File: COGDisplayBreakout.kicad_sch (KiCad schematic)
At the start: 12 parts, among them J2 SPI_Header

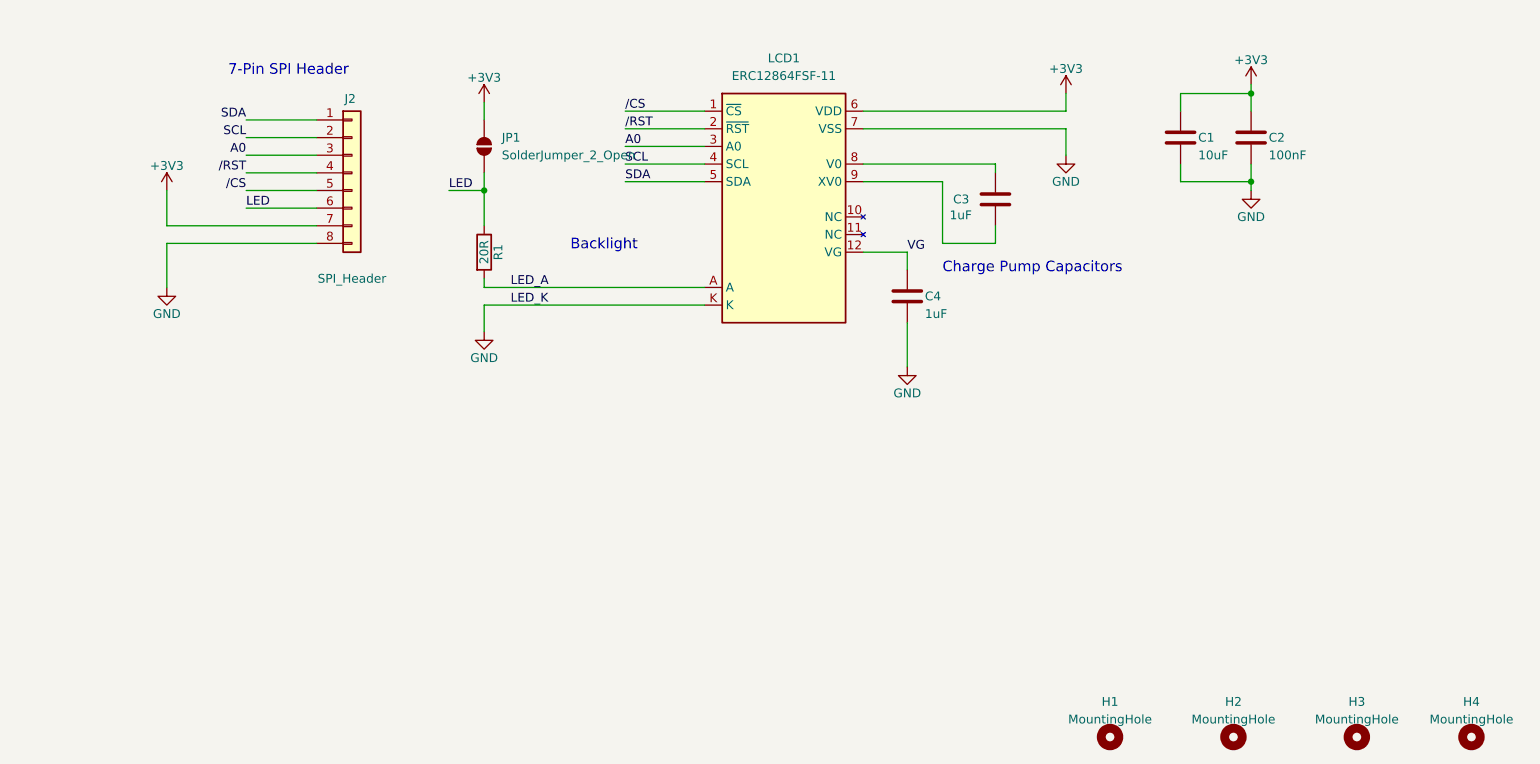
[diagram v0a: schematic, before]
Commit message: readme edits
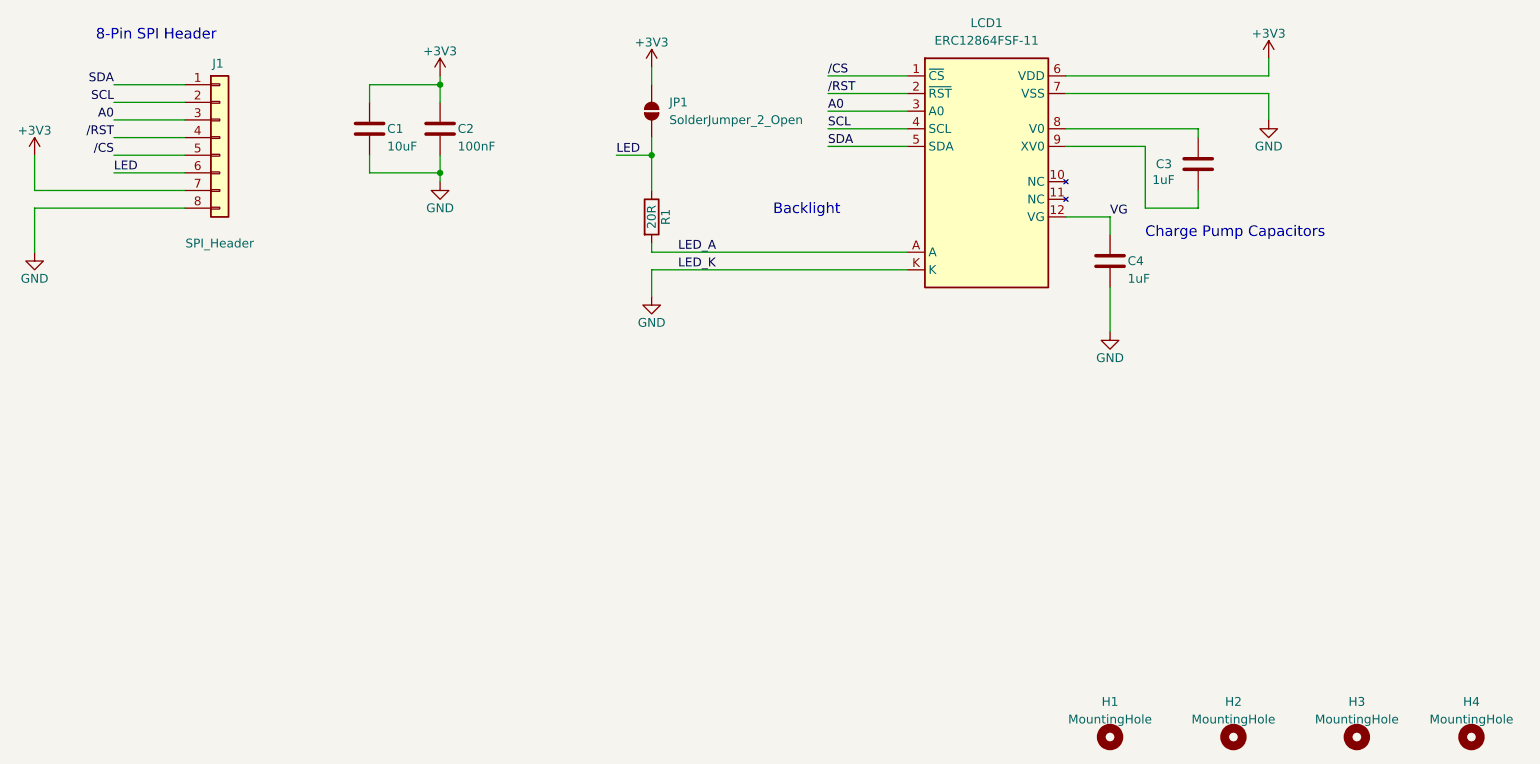
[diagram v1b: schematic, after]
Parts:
- renumbered J2 to J1
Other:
- note added: "8-Pin SPI Header"
- note removed: "7-Pin SPI Header"
- moved on the sheet: C1, C2, C3, C4, J1, JP1, LCD1, R1
